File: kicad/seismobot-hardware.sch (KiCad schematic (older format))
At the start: 36 parts

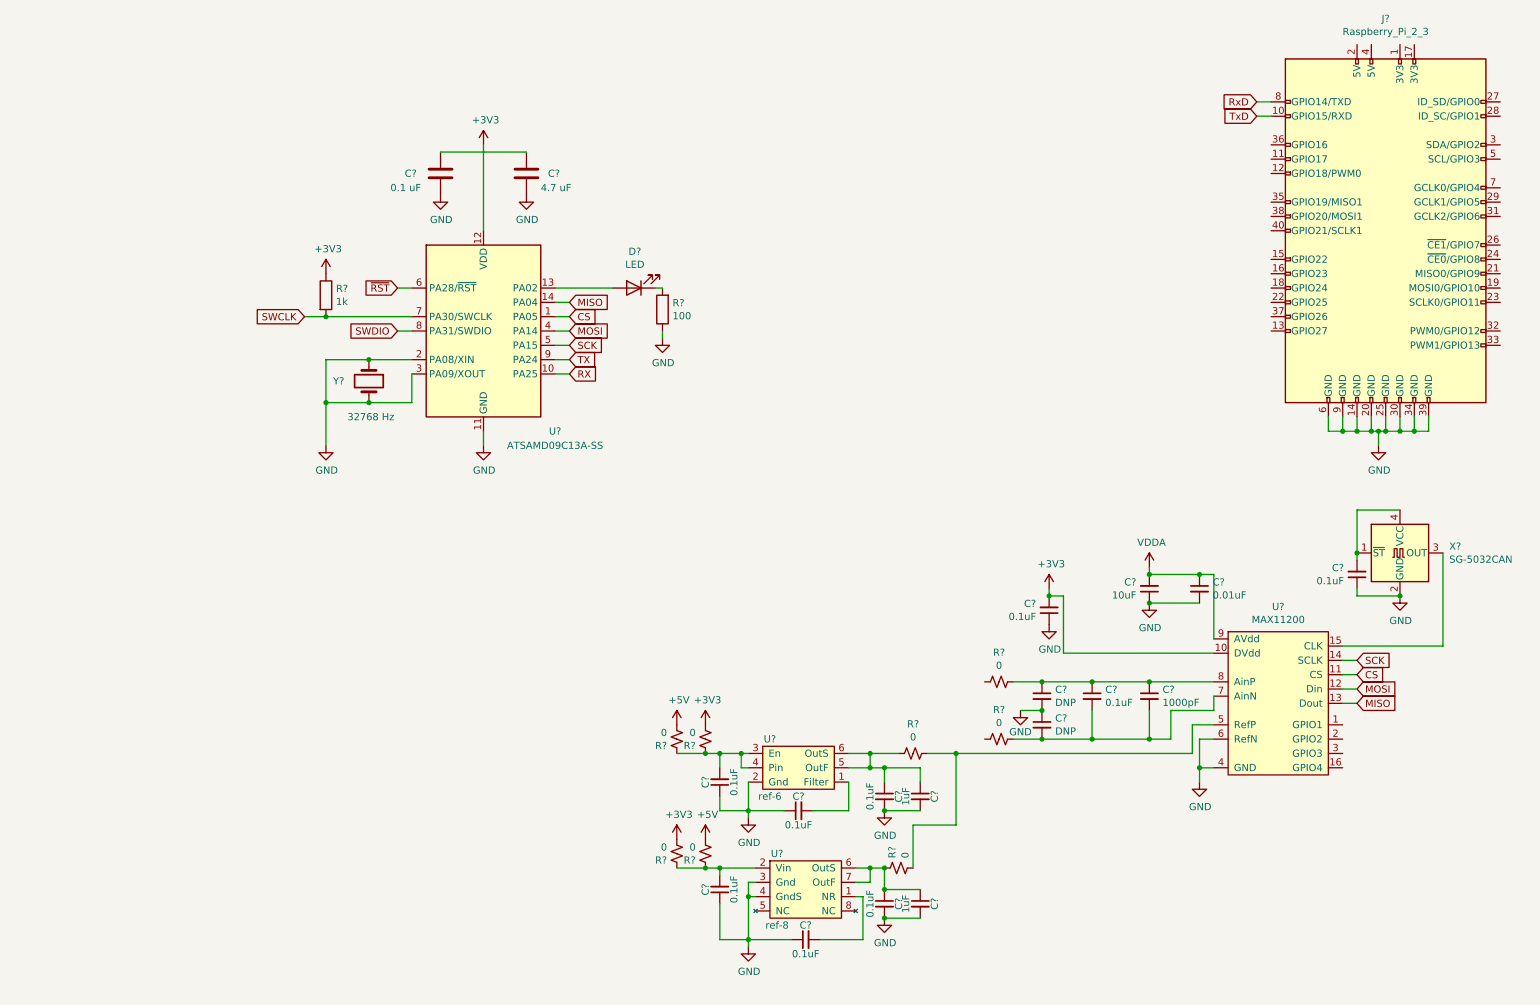
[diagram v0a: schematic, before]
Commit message: add input stage 1
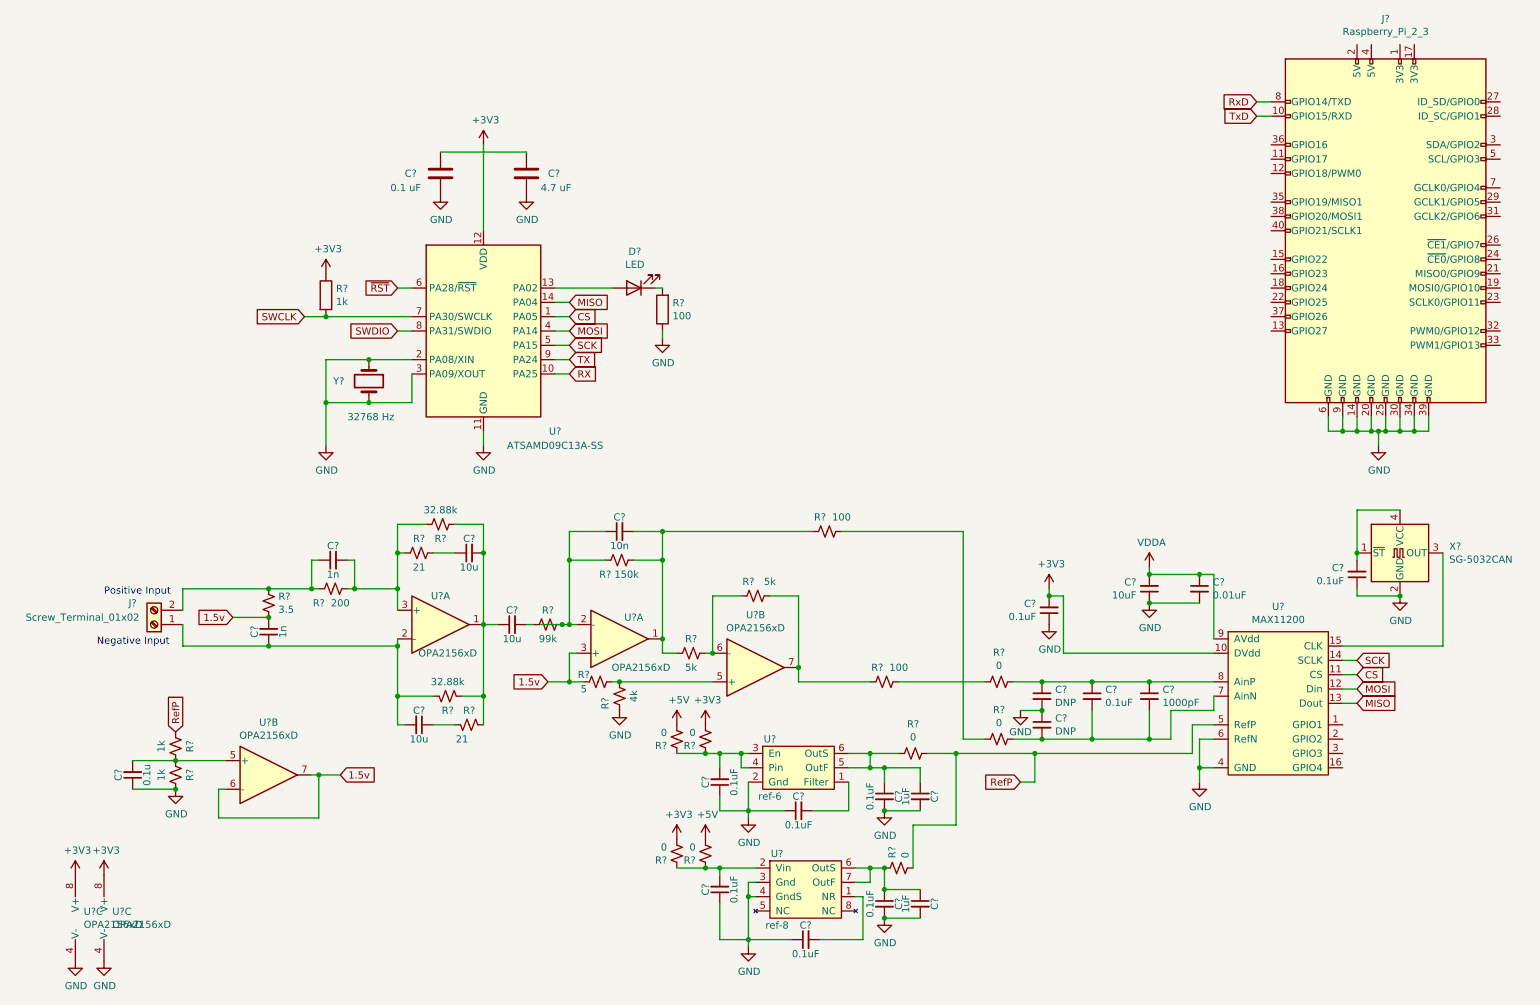
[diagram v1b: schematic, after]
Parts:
- added C? (x2): 1n, symbol Device:C_Small
- added C? (x3): 10u, symbol Device:C_Small
- added C?: 10n, symbol Device:C_Small
- added C?: 0.1u, symbol Device:C_Small
- added J?: Screw_Terminal_01x02, symbol Connector:Screw_Terminal_01x02
- added R?: 3.5, symbol Device:R_Small_US
- added R?: 200, symbol Device:R_Small_US
- added R? (x2): 32.88k, symbol Device:R_Small_US
- added R? (x2): 21, symbol Device:R_Small_US
- added R?: 99k, symbol Device:R_Small_US
- added R?: 150k, symbol Device:R_Small_US
- added R?: 5, symbol Device:R_Small_US
- added R?: 4k, symbol Device:R_Small_US
- added R? (x2): 5k, symbol Device:R_Small_US
- added R? (x2): 100, symbol Device:R_Small_US
- added R? (x2): 1k, symbol Device:R_Small_US
- added U? (x6): OPA2156xD, Package_SO:SOIC-8_3.9x4.9mm_P1.27mm, symbol Amplifier_Operational:OPA2156xD
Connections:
- net +3V3: now also U?.8 (V+), U?.8 (V+)
- net GND: now also C?.1, R?.1, R?.1, U?.4 (V-), U?.4 (V-)
- net RefP: now reaches R?.1, R?.1, U?.5 (RefP)
- net RefP: now also R?.2
- net at R?.2: now also R?.1 (x2)
- new net: C?.1, C?.2, R?.1, R?.2, R?.2, U?.1
- new net: C?.1, C?.2, J?.1 (Pin_1), R?.1, U?.2 (-)
- new net: C?.2, R?.1, R?.2, R?.2, U?.3 (+)
- new net: C?.2, R?.1, R?.2, U?.5 (+)
- new net: C?.1, J?.2 (Pin_2), R?.1, R?.2
- new net: C?.1, R?.1 (x2)
- new net: C?.2, R?.1, R?.2, R?.2, U?.1
- new net: C?.1, R?.1, R?.2, U?.2 (-)
- new net: C?.2, R?.2
- new net: R?.1, R?.2, U?.5 (+)
- new net: R?.1, R?.2, U?.6 (-)
- new net: R?.1, R?.2, U?.7
- new net 1.5v: C?.2, R?.2, R?.2, U?.3 (+), U?.6 (-), U?.7
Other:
- note added: "Negative Input"
- note added: "Positive Input"
